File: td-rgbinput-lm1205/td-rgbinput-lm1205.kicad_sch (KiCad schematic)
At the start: 10 parts, among them J16 Conn_01x06_Male, J2 Conn_01x07_Male, J3 Conn_01x05_Pin, U1 AP2204K-3.3

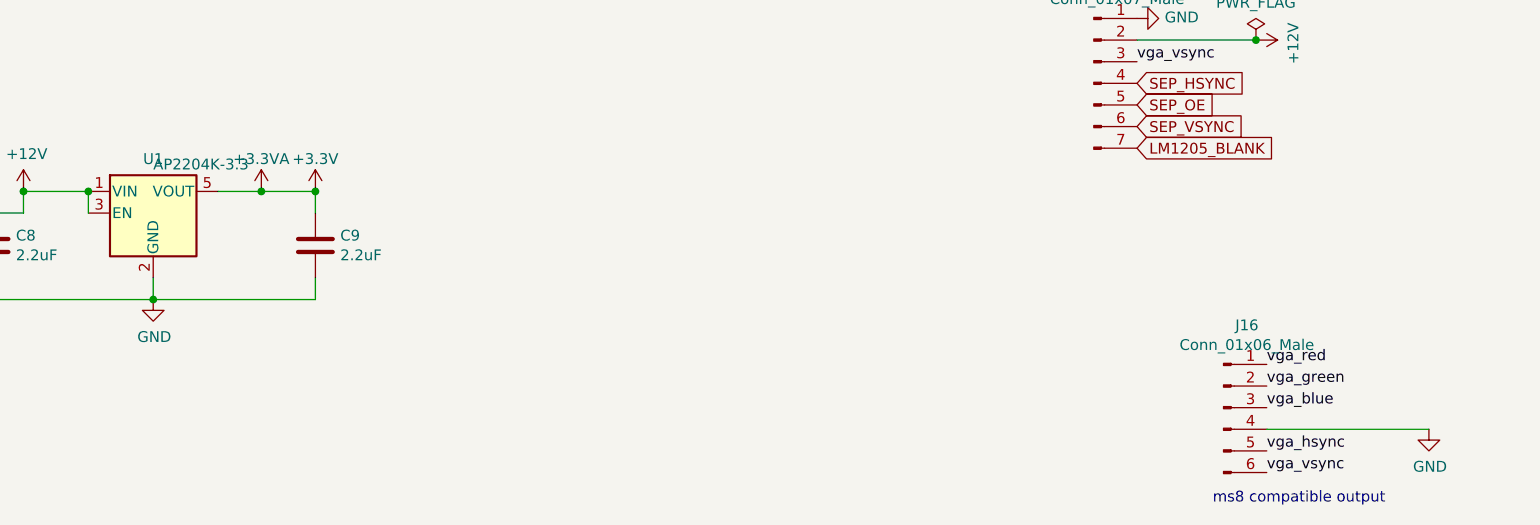
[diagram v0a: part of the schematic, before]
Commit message: update lm1205 to v1.0
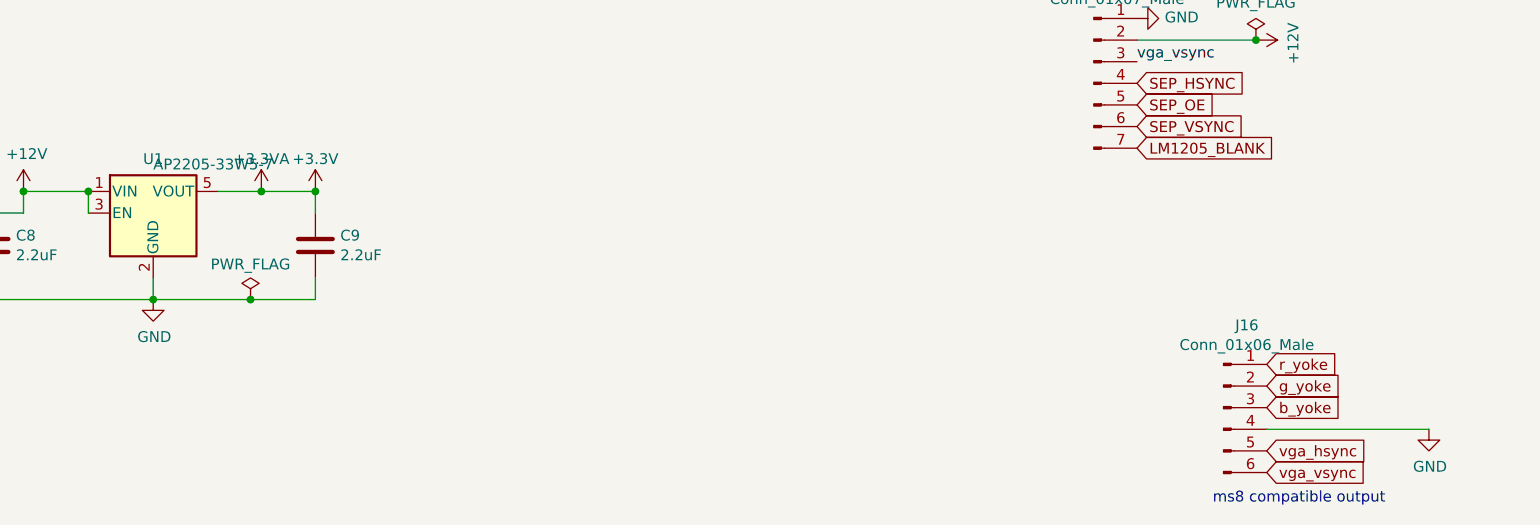
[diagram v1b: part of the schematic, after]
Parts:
- J2: footprint Connector_JST:JST_XH_B7B-XH-AM_1x07_P2.50mm_Vertical -> Connector_JST:JST_XH_B7B-XH-A_1x07_P2.50mm_Vertical
- J3: Digikey (none) -> B5B-XH-A
- U1: value AP2204K-3.3 -> AP2205-33W5-7; Digikey (none) -> 31-AP2205-33W5-7CT-ND
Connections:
- net vga_blue renamed b_yoke
- net vga_green renamed g_yoke
- net vga_red renamed r_yoke
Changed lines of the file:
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@@
   (junction (at 129.54 228.6) (diameter 0) (color 0 0 0 0)
   )
+  (junction (at 140.97 228.6) (diameter 0) (color 0 0 0 0)
+  )
   (junction (at 114.3 215.9) (diameter 0) (color 0 0 0 0)
   )
@@
   )
   (junction (at 322.58 229.87) (diameter 0) (color 0 0 0 0)
+  )
+  (wire (pts (xy 140.97 228.6) (xy 148.59 228.6))
+    (stroke (width 0) (type default))
   )
   (wire (pts (xy 114.3 215.9) (xy 121.92 215.9))
@@
     (stroke (width 0) (type default))
   )
-  (wire (pts (xy 129.54 228.6) (xy 148.59 228.6))
+  (wire (pts (xy 129.54 228.6) (xy 140.97 228.6))
     (stroke (width 0) (type default))
   )
@@
     (effects (font (size 1.27 1.27)) (justify left bottom))
   )
-  (label "vga_vsync" (at 260.35 248.92 0) (fields_autoplaced)
-    (effects (font (size 1.27 1.27)) (justify left bottom))
-  )
   (label "vga_vsync" (at 245.11 200.66 0) (fields_autoplaced)
     (effects (font (size 1.27 1.27)) (justify left bottom))
   )
-  (label "vga_green" (at 260.35 238.76 0) (fields_autoplaced)
-    (effects (font (size 1.27 1.27)) (justify left bottom))
-  )
-  (label "vga_red" (at 260.35 236.22 0) (fields_autoplaced)
-    (effects (font (size 1.27 1.27)) (justify left bottom))
-  )
-  (label "vga_hsync" (at 260.35 246.38 0) (fields_autoplaced)
-    (effects (font (size 1.27 1.27)) (justify left bottom))
-  )
-  (label "vga_blue" (at 260.35 241.3 0) (fields_autoplaced)
-    (effects (font (size 1.27 1.27)) (justify left bottom))
+  (global_label "b_yoke" (shape input) (at 260.35 241.3 0) (fields_autoplaced)
+    (effects (font (size 1.27 1.27)) (justify left))
+    (property "Intersheetrefs" "${INTERSHEET_REFS}" (at 269.0309 241.3 0)
+      (effects (font (size 1.27 1.27)) (justify left) hide)
+    )
   )
   (global_label "GAIN_LOAD" (shape input) (at 148.59 130.81 180) (fields_autoplaced)
@@
     )
   )
+  (global_label "g_yoke" (shape input) (at 260.35 238.76 0) (fields_autoplaced)
+    (effects (font (size 1.27 1.27)) (justify left))
+    (property "Intersheetrefs" "${INTERSHEET_REFS}" (at 269.0309 238.76 0)
+      (effects (font (size 1.27 1.27)) (justify left) hide)
+    )
+  )
+  (global_label "vga_vsync" (shape input) (at 260.35 248.92 0) (fields_autoplaced)
+    (effects (font (size 1.27 1.27)) (justify left))
+    (property "Intersheetrefs" "${INTERSHEET_REFS}" (at 272.1151 248.92 0)
+      (effects (font (size 1.27 1.27)) (justify left) hide)
+    )
+  )
   (global_label "SEP_OE" (shape input) (at 245.11 205.74 0) (fields_autoplaced)
     (effects (font (size 1.27 1.27)) (justify left))
@@
     )
   )
+  (global_label "r_yoke" (shape input) (at 260.35 236.22 0) (fields_autoplaced)
+    (effects (font (size 1.27 1.27)) (justify left))
+    (property "Intersheetrefs" "${INTERSHEET_REFS}" (at 268.6681 236.22 0)
+      (effects (font (size 1.27 1.27)) (justify left) hide)
+    )
+  )
   (global_label "SEP_VSYNC" (shape input) (at 245.11 208.28 0) (fields_autoplaced)
     (effects (font (size 1.27 1.27)) (justify left))
     (property "Intersheetrefs" "${INTERSHEET_REFS}" (at 257.9449 208.28 0)
+      (effects (font (size 1.27 1.27)) (justify left) hide)
+    )
+  )
+  (global_label "vga_hsync" (shape input) (at 260.35 246.38 0) (fields_autoplaced)
+    (effects (font (size 1.27 1.27)) (justify left))
+    (property "Intersheetrefs" "${INTERSHEET_REFS}" (at 272.2965 246.38 0)
       (effects (font (size 1.27 1.27)) (justify left) hide)
     )
@@
       (effects (font (size 1.27 1.27)))
     )
-    (property "Footprint" "Connector_JST:JST_XH_B7B-XH-AM_1x07_P2.50mm_Vertical" (at 240.03 203.2 0)
+    (property "Footprint" "Connector_JST:JST_XH_B7B-XH-A_1x07_P2.50mm_Vertical" (at 240.03 203.2 0)
       (effects (font (size 1.27 1.27)) hide)
     )
@@
       (effects (font (size 1.27 1.27)) hide)
     )
+    (property "Digikey" "B5B-XH-A" (at 153.67 128.27 0)
+      (effects (font (size 1.27 1.27)) hide)
+    )
     (pin "1")
     (pin "2")
@@
       (effects (font (size 1.27 1.27)))
     )
-    (property "Value" "AP2204K-3.3" (at 129.54 212.725 0)
+    (property "Value" "AP2205-33W5-7" (at 129.54 212.725 0)
       (effects (font (size 1.27 1.27)) (justify left))
     )
@@
     )
     (property "Datasheet" "https://www.diodes.com/assets/Datasheets/AP2204.pdf" (at 129.54 215.9 0)
+      (effects (font (size 1.27 1.27)) hide)
+    )
+    (property "Digikey" "31-AP2205-33W5-7CT-ND" (at 129.54 218.44 0)
       (effects (font (size 1.27 1.27)) hide)
     )
@@
     )
   )
-  (symbol (lib_name "GND_1") (lib_id "power:GND") (at 148.59 133.35 270) (unit 1)
+  (symbol (lib_id "power:GND") (at 148.59 133.35 270) (unit 1)
     (in_bom yes) (on_board yes) (dnp no) (fields_autoplaced)
     (property "Reference" "#PWR06" (at 142.24 133.35 0)
@@
         )
       )
+    )
+  )
+  (symbol (lib_id "power:PWR_FLAG") (at 140.97 228.6 0) (unit 1)
+    (in_bom yes) (on_board yes) (dnp no) (fields_autoplaced)
+    (property "Reference" "#FLG01" (at 140.97 226.695 0)
+      (effects (font (size 1.27 1.27)) hide)
+    )
+    (property "Value" "PWR_FLAG" (at 140.97 224.4669 0)
+      (effects (font (size 1.27 1.27)))
+    )
+    (property "Footprint" "" (at 140.97 228.6 0)
+      (effects (font (size 1.27 1.27)) hide)
+    )
+    (property "Datasheet" "~" (at 140.97 228.6 0)
+      (effects (font (size 1.27 1.27)) hide)
+    )
+    (pin "1")
+    (instances
+      (project "td-rgbinput-lm1205"
+        (path "/3efa2ece-8f3f-4a8c-96e9-6ab3ec6f1f70"
+          (reference "#FLG01") (unit 1)
+        )
+      )
